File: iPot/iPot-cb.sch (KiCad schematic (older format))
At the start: 40 parts, among them CON1 12VDC, IC1 ATMEGA644-P, P1 JTAG, P10 SPRAY_PUMP, P11 USB_PWR, P2 SPI, P3 UART, P4 SOIL, P5 TEMP/HUMID, P6 LIGHT, P7 WATER_TANK, P8 POT_BASE, P9 WATER_PUMP, Q1 IRF630, Q2 IRF630, Q3 2SC1815, Q4 2SC1815, Q5 2SC1815, Q6 2SC1815, SW1 RESET_SW, Y1 10MHz

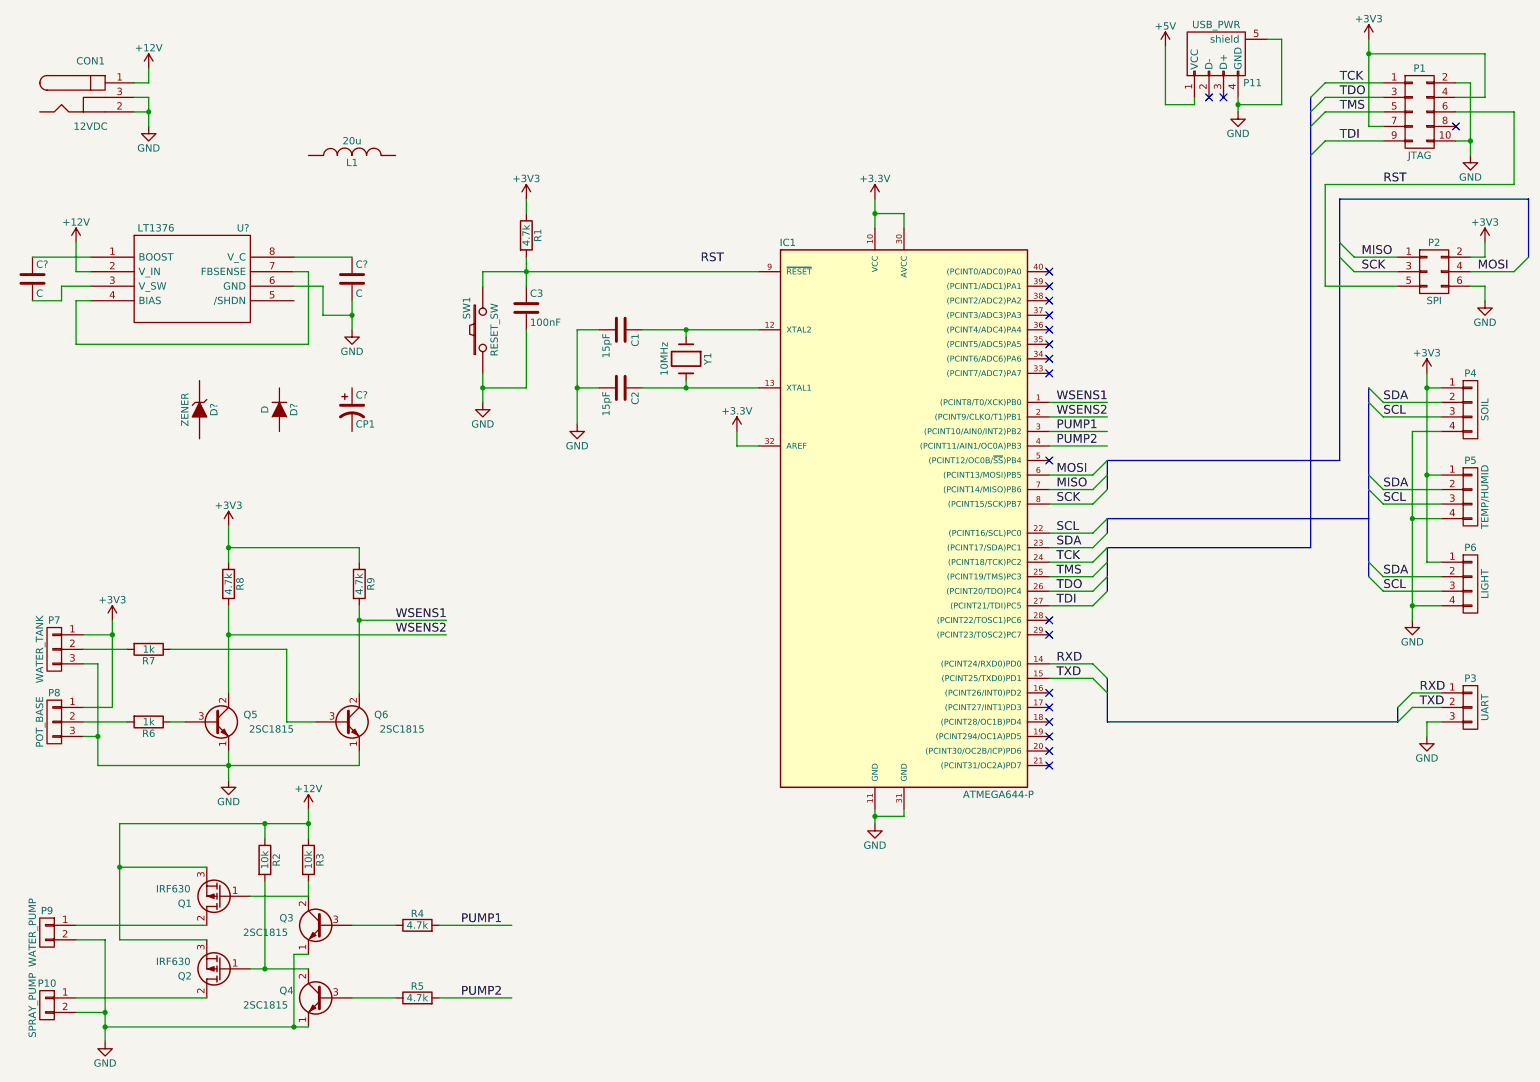
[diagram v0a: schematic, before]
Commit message: Design draft complete
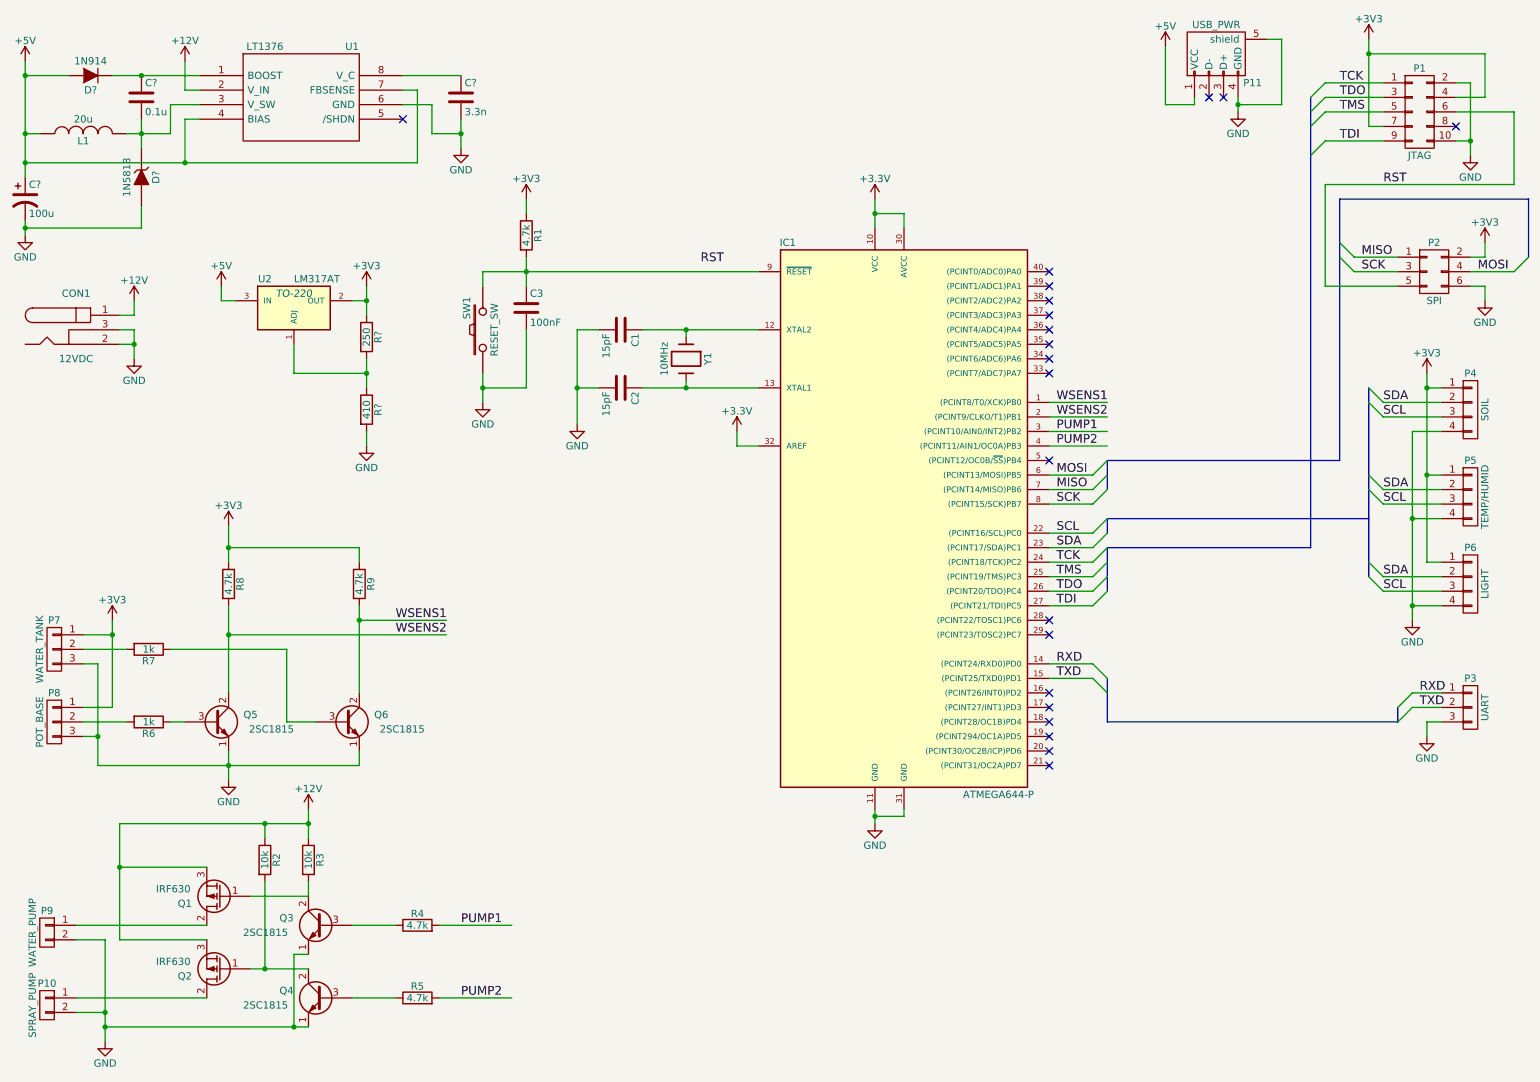
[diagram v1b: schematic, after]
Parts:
- added R?: 410, symbol R
- added R?: 250, symbol R
- added U2: LM317AT, TO-220, symbol LM317AT
- C?: value C -> 0.1u
- C?: value C -> 3.3n
- C?: value CP1 -> 100u
- D?: value ZENER -> 1N5818
- D?: value D -> 1N914
- gave numbers to parts that had none: 1
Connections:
- wire segments 151 -> 207
- no-connect marks 20 -> 21
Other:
- moved on the sheet: C?, CON1, D?, L1, U1
